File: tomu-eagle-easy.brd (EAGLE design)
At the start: 24.8 x 10.2 mm, 18 parts, among them U1 EFM32HG309F64G

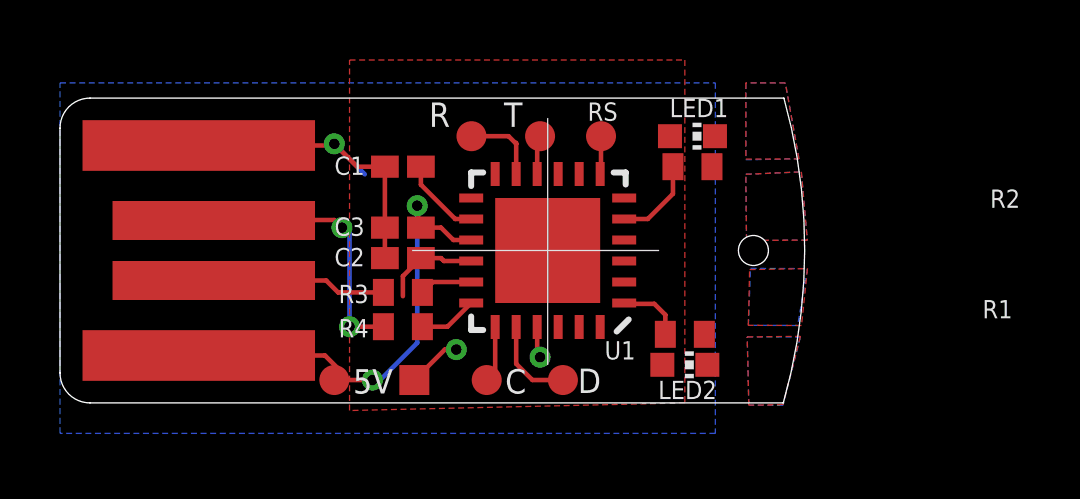
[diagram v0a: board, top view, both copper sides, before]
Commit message: more fixes
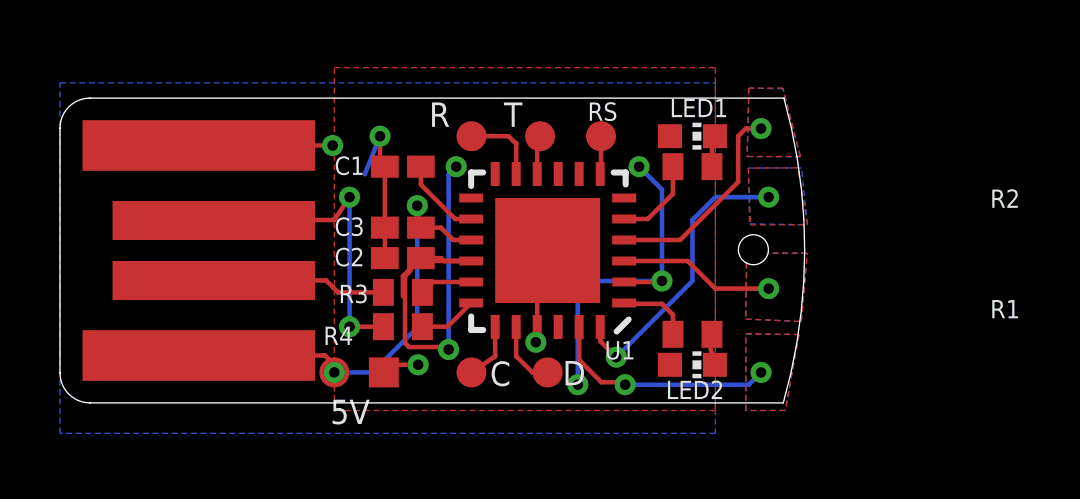
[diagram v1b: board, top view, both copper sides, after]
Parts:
- moved - 1.05 mm to (10.8, 1.78)
- moved C 0.57 mm to (13.7, 1.78)
- moved D 0.57 mm to (16.3, 1.78)
- moved LED2 0.25 mm to (21.1, 2.03)
- moved R1 0.25 mm to (21.1, 3.05)
- moved 5V 0.25 mm to (9.14, 1.78)
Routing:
- net +3V3: track 3.23 -> 26.6 mm, vias 0 -> 5
- net CAP1B: track 0.00 -> 9.71 mm, vias 0 -> 2
- net CAP0B: track 0.00 -> 7.67 mm, vias 0 -> 2
- net CAP1A: track 0.00 -> 7.25 mm, vias 0 -> 1
- net CAP0A: track 0.00 -> 5.20 mm, vias 0 -> 1
- net USB_D+: track 9.32 -> 10.6 mm
- net N$5: track 0.00 -> 1.13 mm
- net N$4: track 0.00 -> 1.06 mm
- net DBG_SWDIO: track 3.01 -> 2.25 mm
- net GND: track 13.9 -> 14.5 mm, vias 3 -> 4
- net VUSB: track 15.9 -> 15.4 mm
